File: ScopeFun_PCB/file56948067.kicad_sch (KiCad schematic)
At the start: 26 parts, among them Q3 BSS138BKS, U12 XC7A35T-FTG256

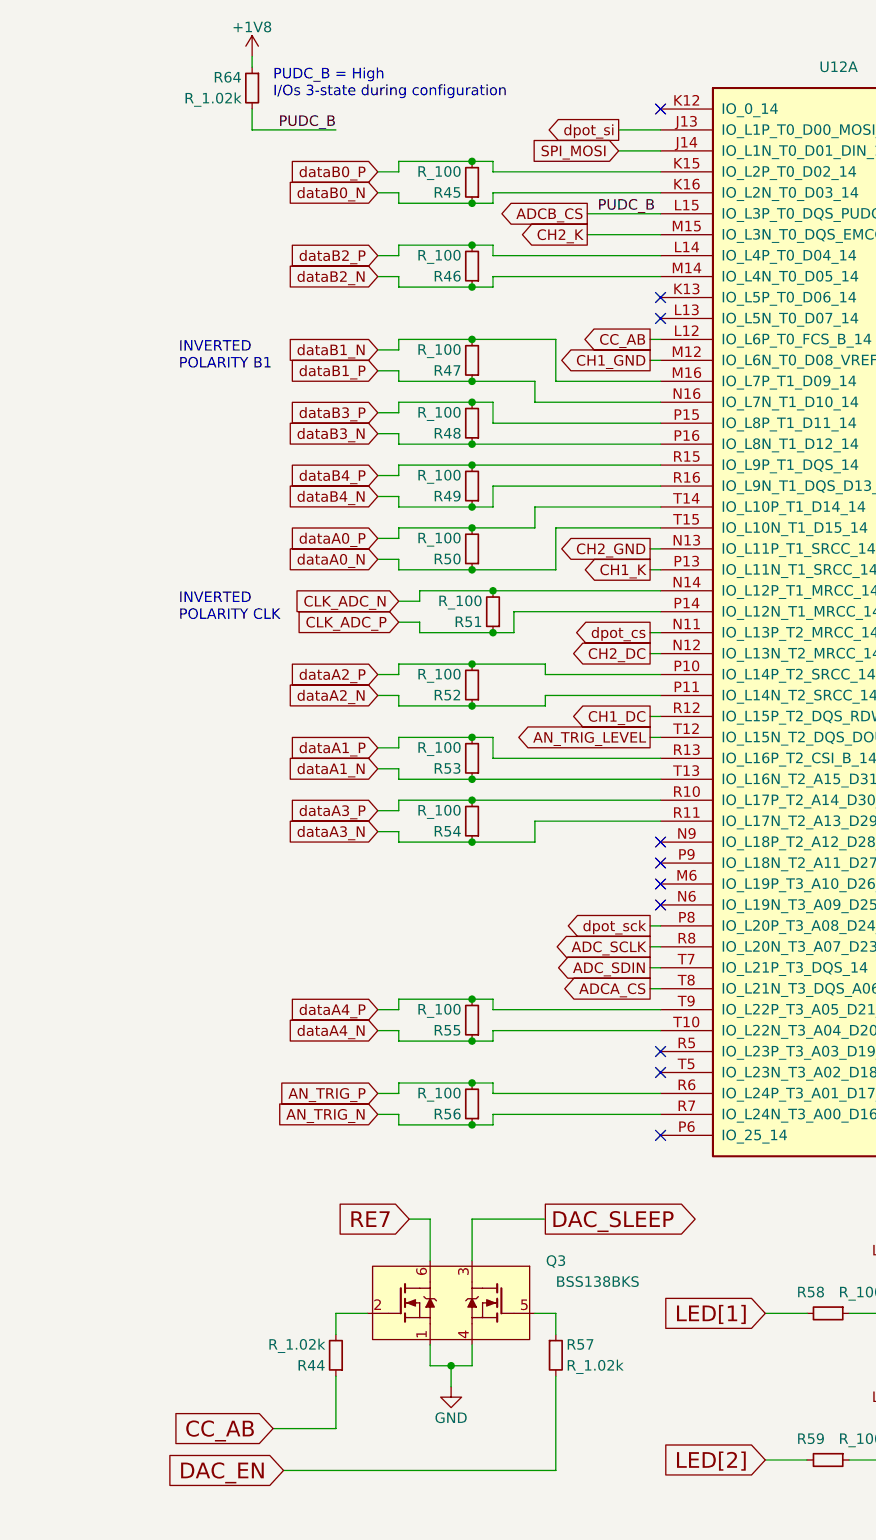
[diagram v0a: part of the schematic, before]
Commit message: 0326
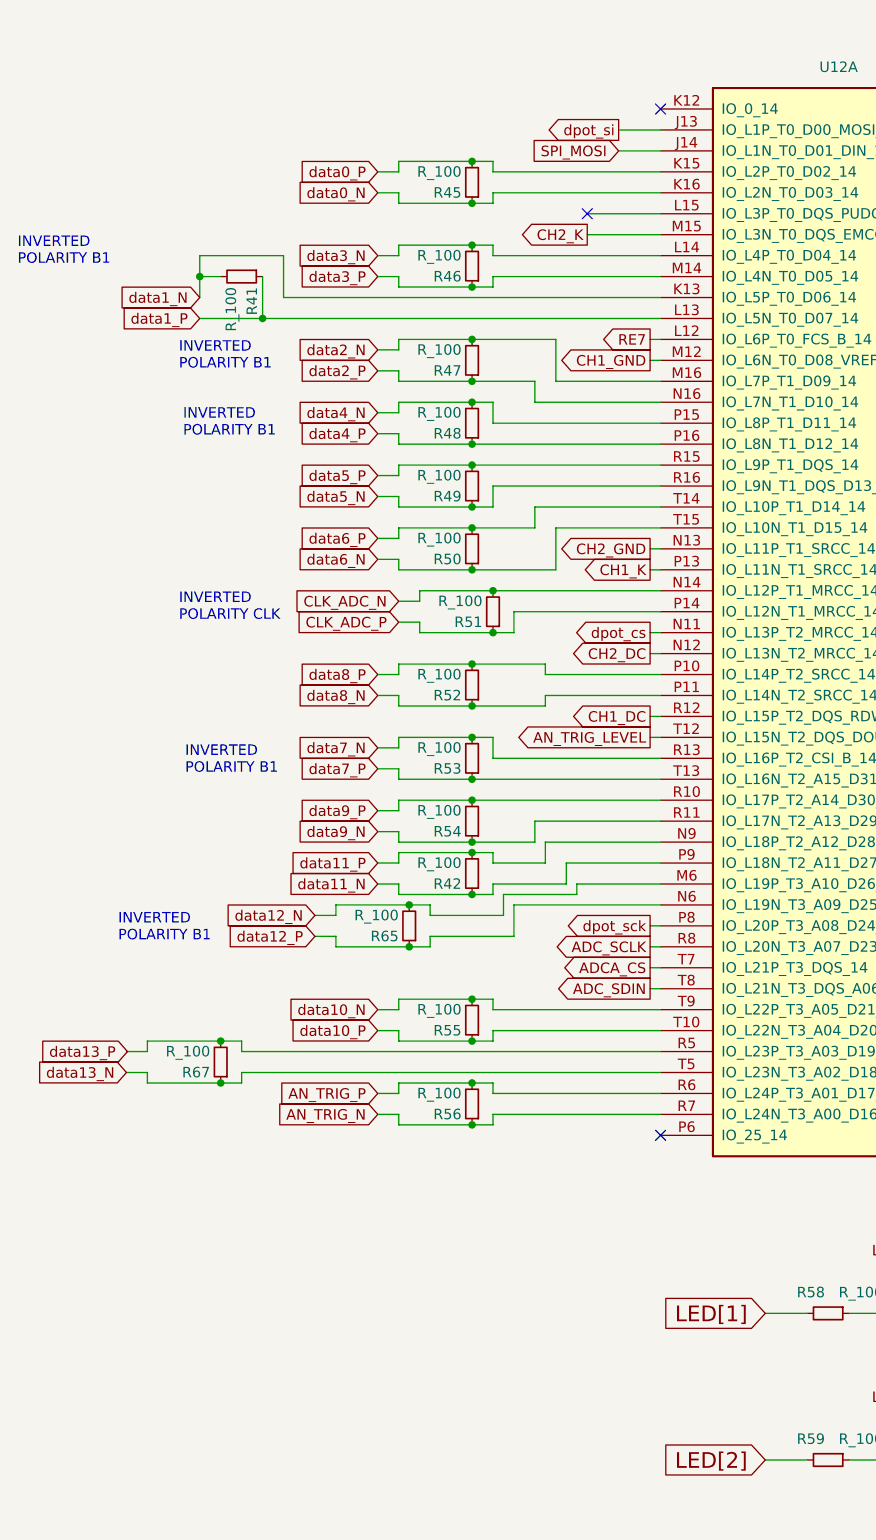
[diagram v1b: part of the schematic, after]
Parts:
- removed Q3: BSS138BKS, ScopefunPackagesLibrary:SOT363, symbol ScopefunParts:BSS138BKS
- removed R44, R57, R64: R_1.02k, ScopefunPackagesLibrary:R_0603, symbol ScopefunParts:R_1.02k
- added R41, R42, R65, R67: R_100, ScopefunPackagesLibrary:R_0402, symbol ScopefunParts:R_100
- SLP1, SLP2, SLP3: footprint ScopefunPackagesLibrary:SLP3-300-100-F -> ScopefunPackagesLibrary:SLP3-300-100-R
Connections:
- net CC_AB is gone; now on net RE7: U12.L12 (IO_L6P_T0_FCS_B_14)
- net ADCA_CS: now also U12.T7 (IO_L21P_T3_DQS_14); no longer U12.T8 (IO_L21N_T3_DQS_A06_D22_14)
- net ADC_SDIN: now also U12.T8 (IO_L21N_T3_DQS_A06_D22_14); no longer U12.T7 (IO_L21P_T3_DQS_14)
- net data1_N: now reaches U12.K13 (IO_L5P_T0_D06_14)
- net data1_N: now also R41.2
- net data1_P: now reaches U12.L13 (IO_L5N_T0_D07_14)
- net data1_P: now also R41.1
- net data12_N: now reaches U12.M6 (IO_L19P_T3_A10_D26_14)
- net data12_N: now also R65.2
- net data12_P: now reaches U12.N6 (IO_L19N_T3_A09_D25_VREF_14)
- net data12_P: now also R65.1
- net data11_P: now reaches U12.N9 (IO_L18P_T2_A12_D28_14)
- net data11_P: now also R42.2
- net data11_N: now reaches U12.P9 (IO_L18N_T2_A11_D27_14)
- net data11_N: now also R42.1
- net data13_P: now reaches U12.R5 (IO_L23P_T3_A03_D19_14)
- net data13_P: now also R67.2
- net data13_N: now reaches U12.T5 (IO_L23N_T3_A02_D18_14)
- net data13_N: now also R67.1
- net ADCB_CS: no longer names the net of U12.L15 (IO_L3P_T0_DQS_PUDC_B_14)
- net dataA0_N renamed data6_N
- net dataA0_P renamed data6_P
- net dataA1_N renamed data7_P
- net dataA1_P renamed data7_N
- net dataA2_N renamed data8_N
- net dataA2_P renamed data8_P
- net dataA3_N renamed data9_N
- net dataA3_P renamed data9_P
- net dataA4_N renamed data10_P
- net dataA4_P renamed data10_N
- net dataB0_N renamed data0_N
- net dataB0_P renamed data0_P
- net dataB1_N renamed data2_N
- net dataB1_P renamed data2_P
- net dataB2_N renamed data3_P
- net dataB2_P renamed data3_N
- net dataB3_N renamed data4_P
- net dataB3_P renamed data4_N
- net dataB4_N renamed data5_N
- net dataB4_P renamed data5_P
- no-connect marks 39 -> 32
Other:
- note removed: "PUDC_B = High I/Os 3-state during configuration"

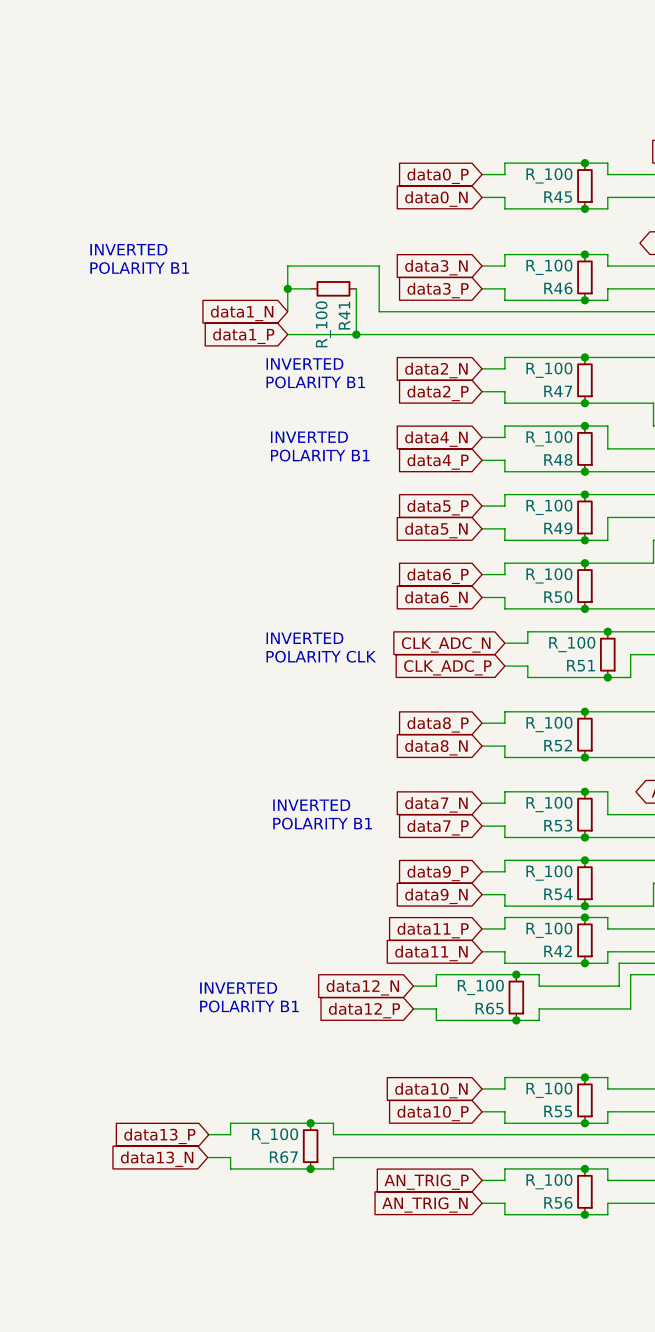
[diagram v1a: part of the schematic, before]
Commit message: 260330
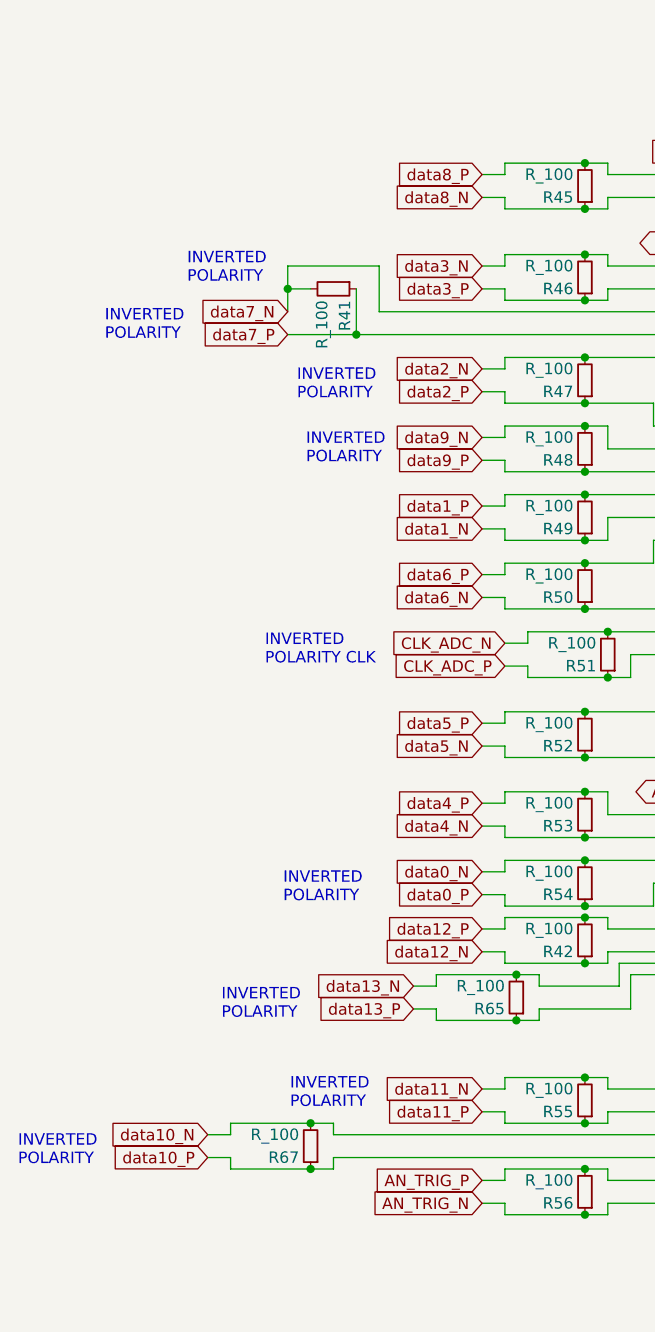
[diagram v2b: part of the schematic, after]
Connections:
- net data0_N: now also R54.2, U12.R10 (IO_L17P_T2_A14_D30_14); no longer R45.1, U12.K16 (IO_L2N_T0_D03_14)
- net data0_P: now also R54.1, U12.R11 (IO_L17N_T2_A13_D29_14); no longer R45.2, U12.K15 (IO_L2P_T0_D02_14)
- net data10_N: now also R67.2, U12.R5 (IO_L23P_T3_A03_D19_14); no longer R55.2, U12.T9 (IO_L22P_T3_A05_D21_14)
- net data10_P: now also R67.1, U12.T5 (IO_L23N_T3_A02_D18_14); no longer R55.1, U12.T10 (IO_L22N_T3_A04_D20_14)
- net data11_N: now also R55.2, U12.T9 (IO_L22P_T3_A05_D21_14); no longer R42.1, U12.P9 (IO_L18N_T2_A11_D27_14)
- net data11_P: now also R55.1, U12.T10 (IO_L22N_T3_A04_D20_14); no longer R42.2, U12.N9 (IO_L18P_T2_A12_D28_14)
- net data12_N: now also R42.1, U12.P9 (IO_L18N_T2_A11_D27_14); no longer R65.2, U12.M6 (IO_L19P_T3_A10_D26_14)
- net data12_P: now also R42.2, U12.N9 (IO_L18P_T2_A12_D28_14); no longer R65.1, U12.N6 (IO_L19N_T3_A09_D25_VREF_14)
- net data13_N: now also R65.2, U12.M6 (IO_L19P_T3_A10_D26_14); no longer R67.1, U12.T5 (IO_L23N_T3_A02_D18_14)
- net data13_P: now also R65.1, U12.N6 (IO_L19N_T3_A09_D25_VREF_14); no longer R67.2, U12.R5 (IO_L23P_T3_A03_D19_14)
- net data1_N: now also R49.1, U12.R16 (IO_L9N_T1_DQS_D13_14); no longer R41.2, U12.K13 (IO_L5P_T0_D06_14)
- net data1_P: now also R49.2, U12.R15 (IO_L9P_T1_DQS_14); no longer R41.1, U12.L13 (IO_L5N_T0_D07_14)
- net data4_N: now also R53.1, U12.T13 (IO_L16N_T2_A15_D31_14); no longer R48.2, U12.P15 (IO_L8P_T1_D11_14)
- net data4_P: now also R53.2, U12.R13 (IO_L16P_T2_CSI_B_14); no longer R48.1, U12.P16 (IO_L8N_T1_D12_14)
- net data5_N: now also R52.1, U12.P11 (IO_L14N_T2_SRCC_14); no longer R49.1, U12.R16 (IO_L9N_T1_DQS_D13_14)
- net data5_P: now also R52.2, U12.P10 (IO_L14P_T2_SRCC_14); no longer R49.2, U12.R15 (IO_L9P_T1_DQS_14)
- net data7_N: now also R41.2, U12.K13 (IO_L5P_T0_D06_14); no longer R53.2, U12.R13 (IO_L16P_T2_CSI_B_14)
- net data7_P: now also R41.1, U12.L13 (IO_L5N_T0_D07_14); no longer R53.1, U12.T13 (IO_L16N_T2_A15_D31_14)
- net data8_N: now also R45.1, U12.K16 (IO_L2N_T0_D03_14); no longer R52.1, U12.P11 (IO_L14N_T2_SRCC_14)
- net data8_P: now also R45.2, U12.K15 (IO_L2P_T0_D02_14); no longer R52.2, U12.P10 (IO_L14P_T2_SRCC_14)
- net data9_N: now also R48.2, U12.P15 (IO_L8P_T1_D11_14); no longer R54.1, U12.R11 (IO_L17N_T2_A13_D29_14)
- net data9_P: now also R48.1, U12.P16 (IO_L8N_T1_D12_14); no longer R54.2, U12.R10 (IO_L17P_T2_A14_D30_14)
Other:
- note added: "INVERTED POLARITY"
- note removed: "INVERTED POLARITY B1"

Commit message: 1
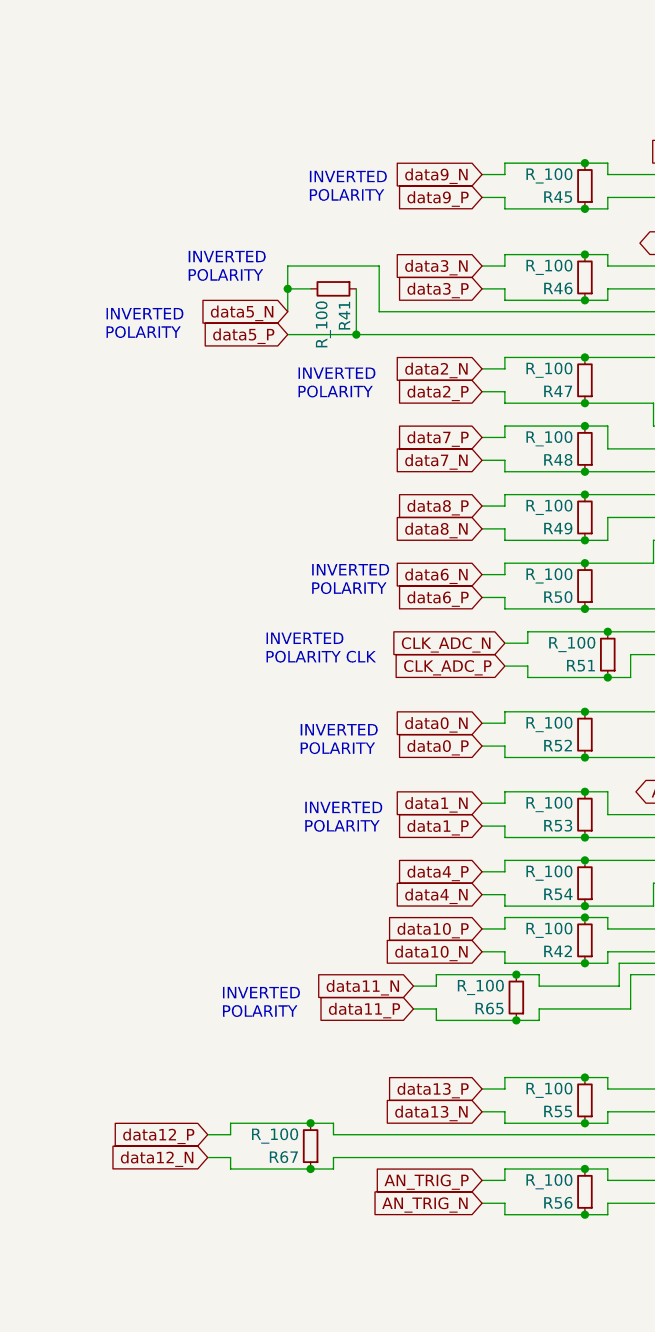
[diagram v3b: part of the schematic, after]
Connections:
- net data0_N: now also R52.2, U12.P10 (IO_L14P_T2_SRCC_14); no longer R54.2, U12.R10 (IO_L17P_T2_A14_D30_14)
- net data0_P: now also R52.1, U12.P11 (IO_L14N_T2_SRCC_14); no longer R54.1, U12.R11 (IO_L17N_T2_A13_D29_14)
- net data10_N: now also R42.1, U12.P9 (IO_L18N_T2_A11_D27_14); no longer R67.2, U12.R5 (IO_L23P_T3_A03_D19_14)
- net data10_P: now also R42.2, U12.N9 (IO_L18P_T2_A12_D28_14); no longer R67.1, U12.T5 (IO_L23N_T3_A02_D18_14)
- net data11_N: now also R65.2, U12.M6 (IO_L19P_T3_A10_D26_14); no longer R55.2, U12.T9 (IO_L22P_T3_A05_D21_14)
- net data11_P: now also R65.1, U12.N6 (IO_L19N_T3_A09_D25_VREF_14); no longer R55.1, U12.T10 (IO_L22N_T3_A04_D20_14)
- net data12_N: now also R67.1, U12.T5 (IO_L23N_T3_A02_D18_14); no longer R42.1, U12.P9 (IO_L18N_T2_A11_D27_14)
- net data12_P: now also R67.2, U12.R5 (IO_L23P_T3_A03_D19_14); no longer R42.2, U12.N9 (IO_L18P_T2_A12_D28_14)
- net data13_N: now also R55.1, U12.T10 (IO_L22N_T3_A04_D20_14); no longer R65.2, U12.M6 (IO_L19P_T3_A10_D26_14)
- net data13_P: now also R55.2, U12.T9 (IO_L22P_T3_A05_D21_14); no longer R65.1, U12.N6 (IO_L19N_T3_A09_D25_VREF_14)
- net data1_N: now also R53.2, U12.R13 (IO_L16P_T2_CSI_B_14); no longer R49.1, U12.R16 (IO_L9N_T1_DQS_D13_14)
- net data1_P: now also R53.1, U12.T13 (IO_L16N_T2_A15_D31_14); no longer R49.2, U12.R15 (IO_L9P_T1_DQS_14)
- net data4_N: now also R54.1, U12.R11 (IO_L17N_T2_A13_D29_14); no longer R53.1, U12.T13 (IO_L16N_T2_A15_D31_14)
- net data4_P: now also R54.2, U12.R10 (IO_L17P_T2_A14_D30_14); no longer R53.2, U12.R13 (IO_L16P_T2_CSI_B_14)
- net data5_N: now also R41.2, U12.K13 (IO_L5P_T0_D06_14); no longer R52.1, U12.P11 (IO_L14N_T2_SRCC_14)
- net data5_P: now also R41.1, U12.L13 (IO_L5N_T0_D07_14); no longer R52.2, U12.P10 (IO_L14P_T2_SRCC_14)
- net data6_N: now also R50.2, U12.T14 (IO_L10P_T1_D14_14); no longer R50.1, U12.T15 (IO_L10N_T1_D15_14)
- net data6_P: now also R50.1, U12.T15 (IO_L10N_T1_D15_14); no longer R50.2, U12.T14 (IO_L10P_T1_D14_14)
- net data7_N: now also R48.1, U12.P16 (IO_L8N_T1_D12_14); no longer R41.2, U12.K13 (IO_L5P_T0_D06_14)
- net data7_P: now also R48.2, U12.P15 (IO_L8P_T1_D11_14); no longer R41.1, U12.L13 (IO_L5N_T0_D07_14)
- net data8_N: now also R49.1, U12.R16 (IO_L9N_T1_DQS_D13_14); no longer R45.1, U12.K16 (IO_L2N_T0_D03_14)
- net data8_P: now also R49.2, U12.R15 (IO_L9P_T1_DQS_14); no longer R45.2, U12.K15 (IO_L2P_T0_D02_14)
- net data9_N: now also R45.2, U12.K15 (IO_L2P_T0_D02_14); no longer R48.2, U12.P15 (IO_L8P_T1_D11_14)
- net data9_P: now also R45.1, U12.K16 (IO_L2N_T0_D03_14); no longer R48.1, U12.P16 (IO_L8N_T1_D12_14)

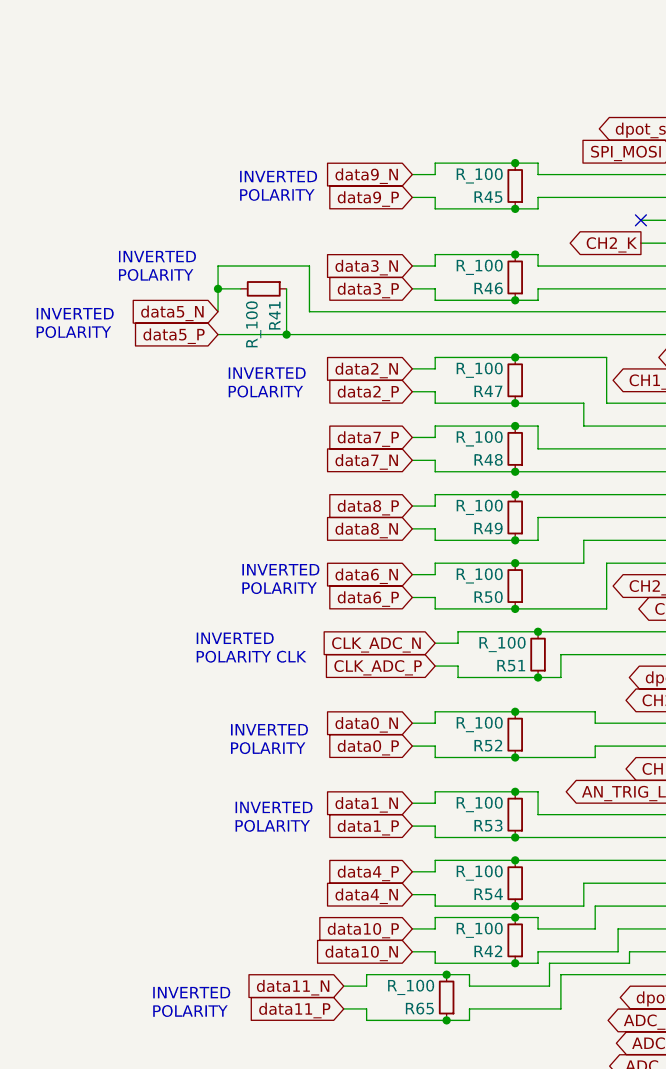
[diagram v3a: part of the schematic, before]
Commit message: 260407
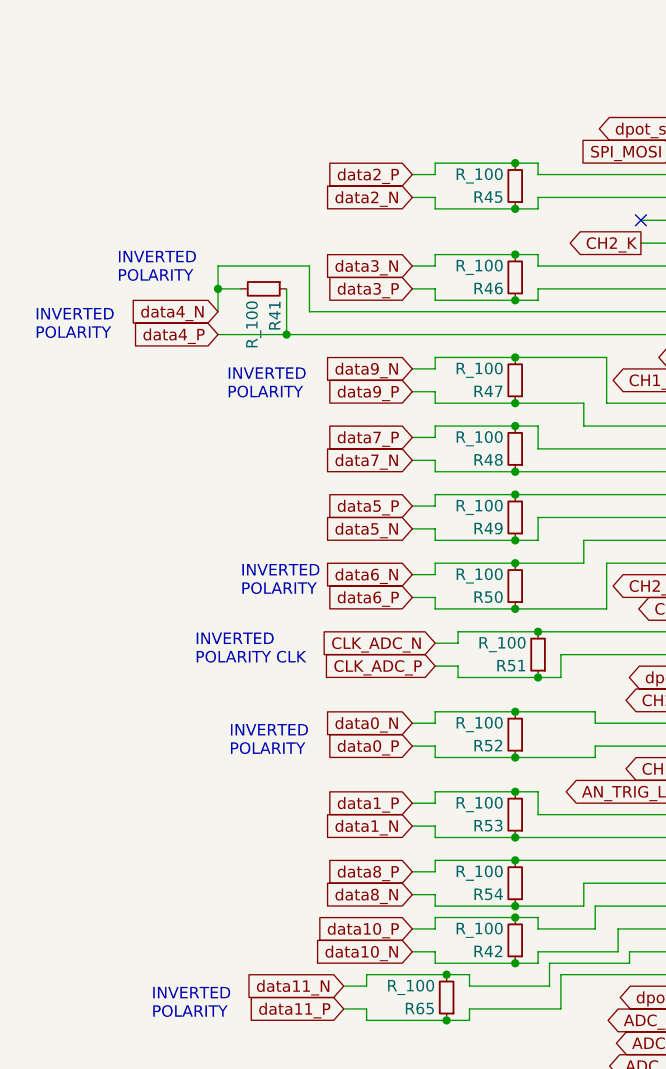
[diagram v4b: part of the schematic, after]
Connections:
- net data1_N: now also R53.1, U12.T13 (IO_L16N_T2_A15_D31_14); no longer R53.2, U12.R13 (IO_L16P_T2_CSI_B_14)
- net data1_P: now also R53.2, U12.R13 (IO_L16P_T2_CSI_B_14); no longer R53.1, U12.T13 (IO_L16N_T2_A15_D31_14)
- net data2_N: now also R45.1, U12.K16 (IO_L2N_T0_D03_14); no longer R47.2, U12.M16 (IO_L7P_T1_D09_14)
- net data2_P: now also R45.2, U12.K15 (IO_L2P_T0_D02_14); no longer R47.1, U12.N16 (IO_L7N_T1_D10_14)
- net data4_N: now also R41.2, U12.K13 (IO_L5P_T0_D06_14); no longer R54.1, U12.R11 (IO_L17N_T2_A13_D29_14)
- net data4_P: now also R41.1, U12.L13 (IO_L5N_T0_D07_14); no longer R54.2, U12.R10 (IO_L17P_T2_A14_D30_14)
- net data5_N: now also R49.1, U12.R16 (IO_L9N_T1_DQS_D13_14); no longer R41.2, U12.K13 (IO_L5P_T0_D06_14)
- net data5_P: now also R49.2, U12.R15 (IO_L9P_T1_DQS_14); no longer R41.1, U12.L13 (IO_L5N_T0_D07_14)
- net data8_N: now also R54.1, U12.R11 (IO_L17N_T2_A13_D29_14); no longer R49.1, U12.R16 (IO_L9N_T1_DQS_D13_14)
- net data8_P: now also R54.2, U12.R10 (IO_L17P_T2_A14_D30_14); no longer R49.2, U12.R15 (IO_L9P_T1_DQS_14)
- net data9_N: now also R47.2, U12.M16 (IO_L7P_T1_D09_14); no longer R45.2, U12.K15 (IO_L2P_T0_D02_14)
- net data9_P: now also R47.1, U12.N16 (IO_L7N_T1_D10_14); no longer R45.1, U12.K16 (IO_L2N_T0_D03_14)
